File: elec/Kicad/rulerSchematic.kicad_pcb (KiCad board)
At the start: 2 copper layers, 30.1 x 155 mm, 121 parts, among them J1 USART, J2 B2B-XH-A, J3 HX0201800000G, J4 Conn_01x05, J5 TestPoint, J6 SWD, J7 USB_B_Micro_MAIN, J8 SD_CARD_CONN, J9 Conn_01x13, Q1 SI2323DS-T1, Q2 BSS138, Q3 BSS138, Q4 SS8050, Q5 NTK3043NT1G, SW1 SW_Push_Gauche_GO_IN, SW2 SW_Push_Droite_GO_BACK, SW3 SW_Push_Action_LOG_EXIT, SW4 SW_Push_RESET, SW5 SW_Push_BOOT, U1 STM32L053C8T6, U11 MMC5633NJL, U2 BMI160, U3 MCP73831, U4 HTU21D, U5 VL53L0CXV0DH1, U6 MIC5219-2.8YM5, U8 LTR-303ALS-01, U9 TLV62085RLTR, Y1 32MHz, Y2 32.768KHz

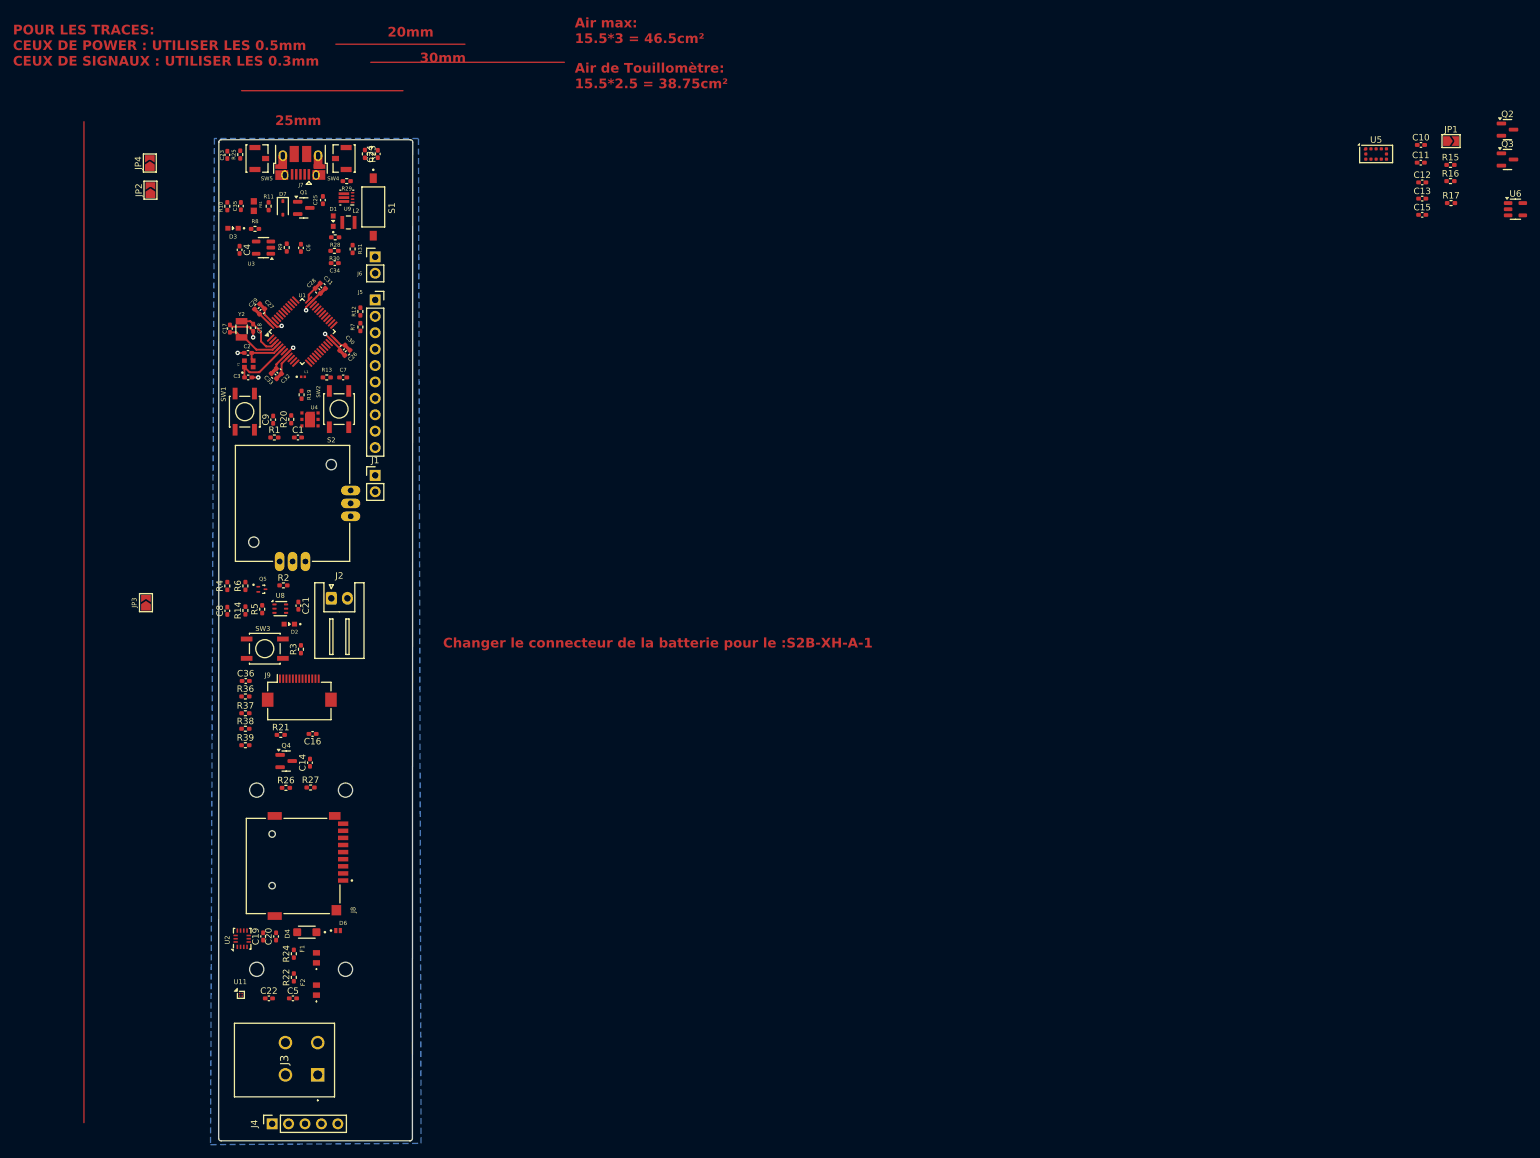
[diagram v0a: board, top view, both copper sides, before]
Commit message: bloatware
fait le slikscree de mesure (merci jabooby)
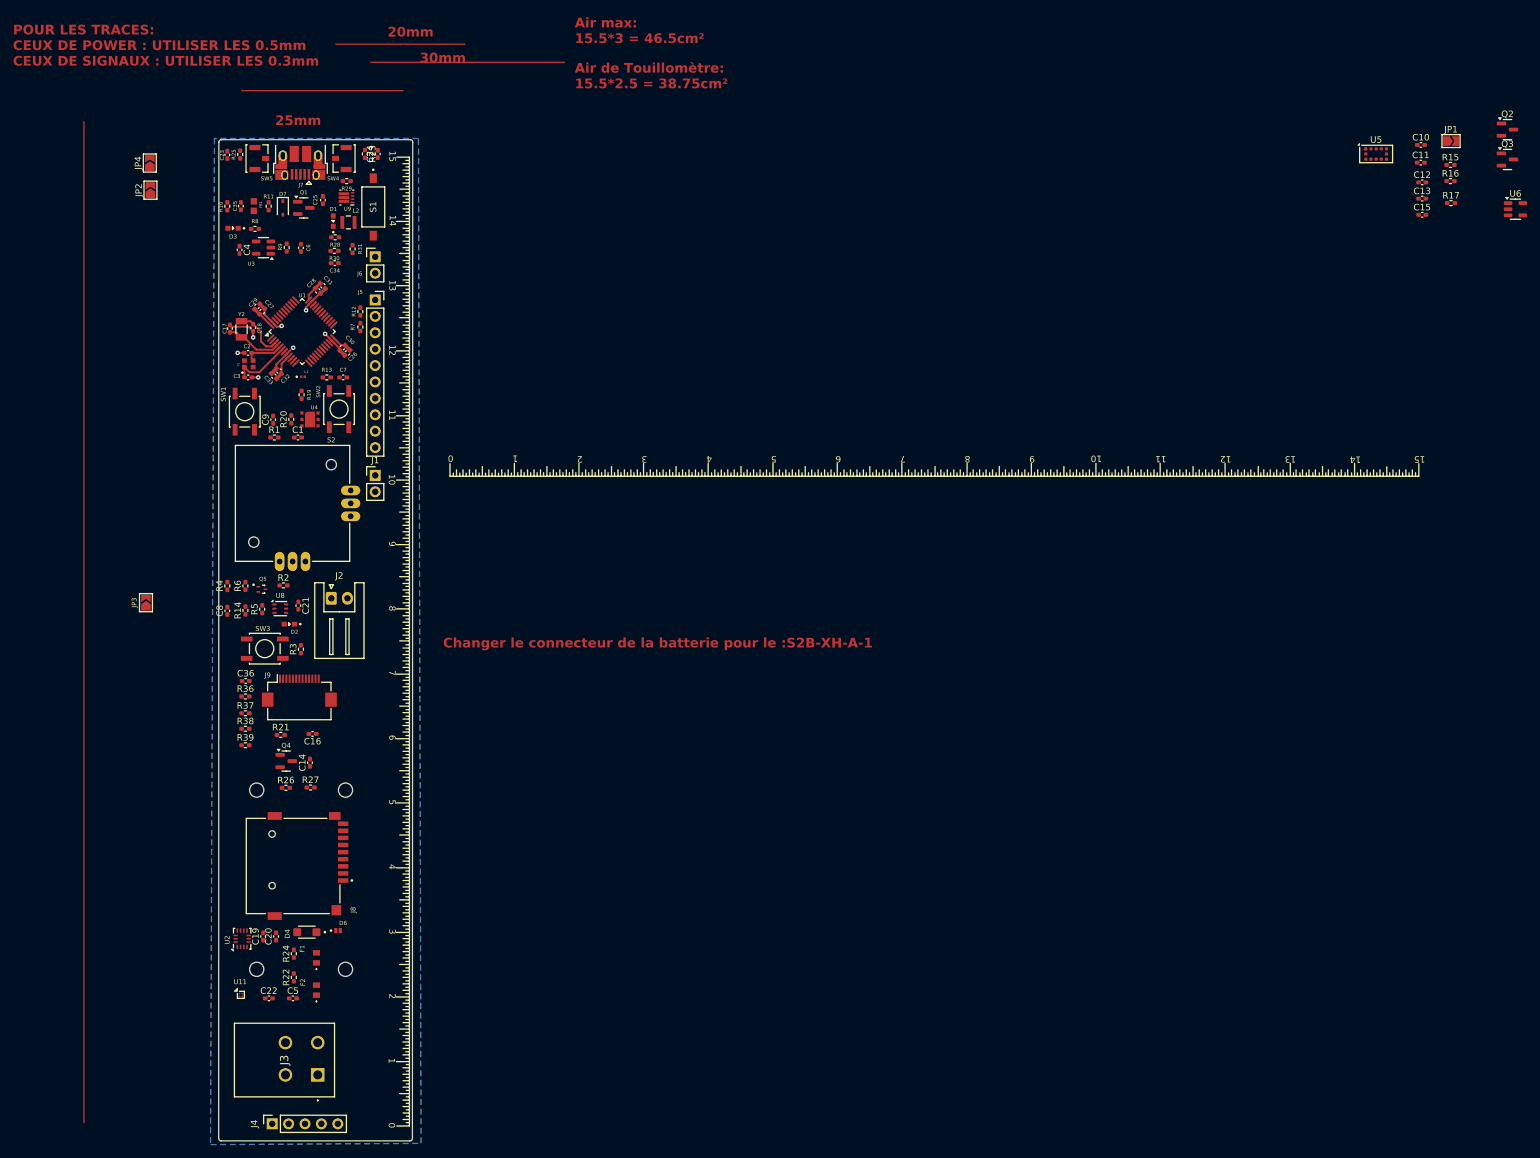
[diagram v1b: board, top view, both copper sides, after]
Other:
- board text added: "0"
- board text added: "1"
- board text added: "10"
- board text added: "11"
- board text added: "12"
- board text added: "13"
- board text added: "14"
- board text added: "15"
- board text added: "2"
- board text added: "3"
- board text added: "4"
- board text added: "5"
- board text added: "6"
- board text added: "7"
- board text added: "8"
- board text added: "9"
